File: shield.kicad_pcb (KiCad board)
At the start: 2 copper layers, 56 parts, among them J1 E5V_Conn, J2 V_SERVO_CONN, P1 ROBOT SELECT, P2 CONN_02X10, P3 ENCODER_TRANS, P4 ENCODER_RIGHT, P5 ENCODER_LEFT, P6 5V_CAN_SELECT, P7 GPIO, Q1 Q_PMOS_DGS, U1 ST_Nucleo144_F429ZI_Morpho, U2 SN65HVD256, U3 SN65HVD256, U4 PCA9685

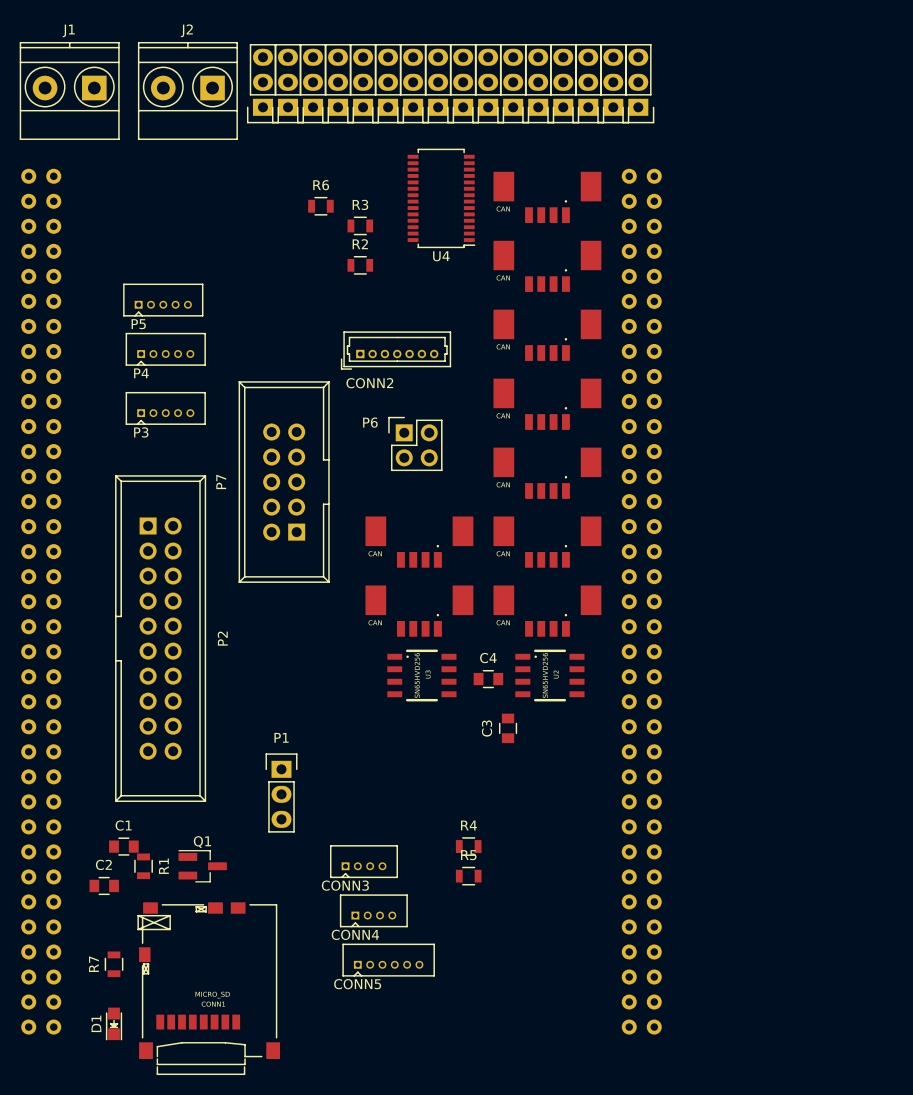
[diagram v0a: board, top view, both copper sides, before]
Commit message: PCB routing
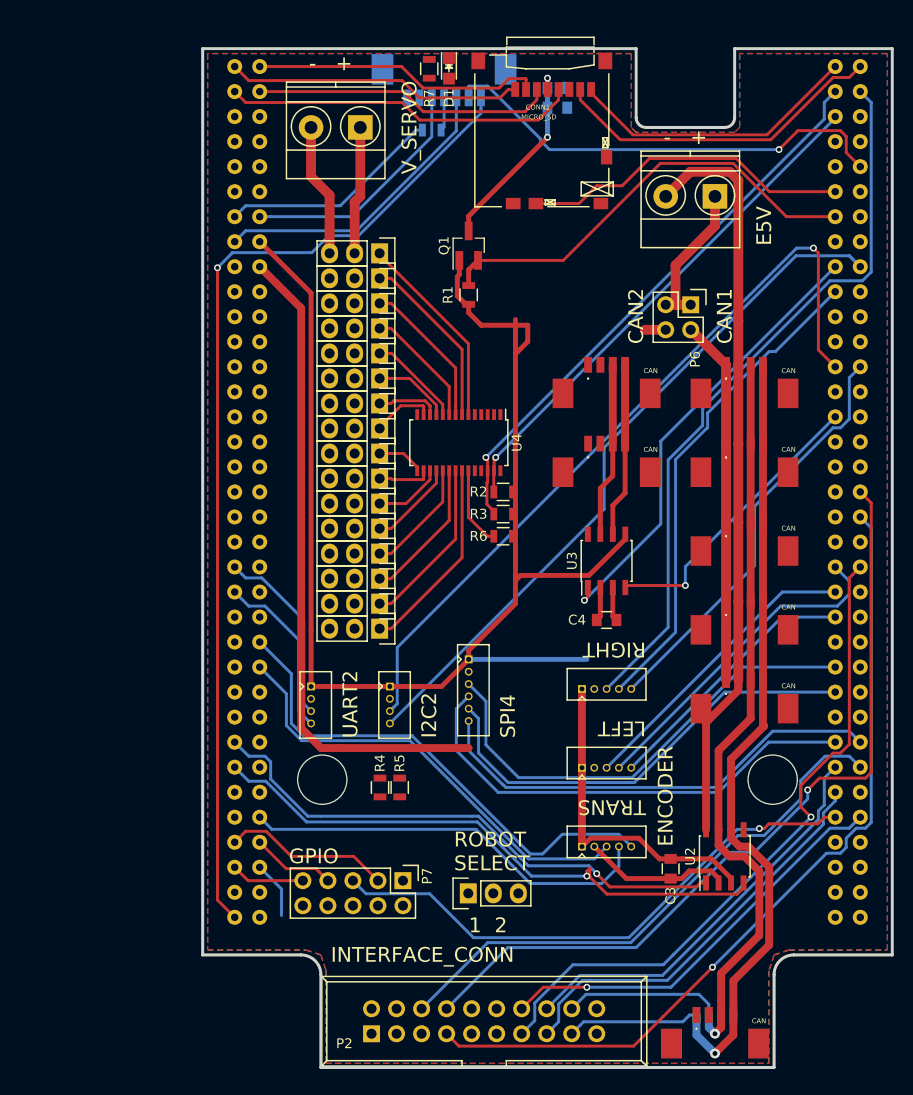
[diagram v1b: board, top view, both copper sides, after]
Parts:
- added R8: 100, Resistors_SMD:R_0805, B.Cu at (88.2, 63.3)
- added _M2: VAL**, _mech:_M2, F.Cu at (122.9, 129.2)
- added _M2: VAL**, _mech:_M2, F.Cu at (77.1, 129.2)
- C1, C2, CONN7: moved to B.Cu
- CONN2: footprint Connectors_Molex:Molex_PicoBlade_53047-0710_07x1.25mm_Straight -> Connectors_Molex:Molex_PicoBlade_53261-0771_07x1.25mm_Angled; moved to B.Cu
- P7: footprint Connect:IDC_Header_Straight_10pins -> Pin_Headers:Pin_Header_Straight_2x05
- U2, U3: footprint _std:_SO-8 -> Housings_SOIC:SOIC-8_3.9x4.9mm_Pitch1.27mm
- moved D1 102.8 mm to (90.0, 57.0), turned to 270 degrees
- moved CONN1 98.8 mm to (96.7, 59.1), turned to 0 degrees
- moved R7 96.4 mm to (88.0, 57.0), turned to 90 degrees
- moved C2 91.4 mm to (101.0, 61.0)
- moved C1 88.7 mm to (101.0, 59.0)
- moved CONN7 81.8 mm to (117.0, 156.0)
- moved CONN8 75.0 mm to (117.0, 156.0), turned to 0 degrees
- moved Q1 68.5 mm to (92.0, 75.0), turned to 90 degrees
- moved R1 66.7 mm to (92.0, 80.0), turned to 90 degrees
- moved P5 65.1 mm to (103.5, 128.0)
- moved J1 64.0 mm to (117.0, 70.0)
- moved P3 62.8 mm to (103.5, 136.0)
- moved P2 56.3 mm to (82.1, 155.0), turned to 0 degrees
- moved P4 56.2 mm to (103.5, 120.0)
- moved CONN30 54.2 mm to (83.0, 113.9), turned to 270 degrees
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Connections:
- CONN2 pad 4: /SWDIO -> Net-(CONN2-Pad4)
- J1 pad 1: GND -> /E5V
- J1 pad 2: /E5V -> GND
- J2 pad 1: GND -> /servo/V_SERVO
- J2 pad 2: /servo/V_SERVO -> GND
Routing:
- net +3.3V: track 0.00 -> 142.3 mm
- net GND: track 0.00 -> 108.1 mm
- net +5V: track 0.00 -> 103.5 mm
- net /DEBUG_UART_RX: track 0.00 -> 101.5 mm, vias 0 -> 1
- net /CAN1L: track 0.00 -> 93.9 mm, vias 0 -> 1
- net /CAN1H: track 0.00 -> 91.9 mm, vias 0 -> 1
- net /EXT_IO_4: track 0.00 -> 85.0 mm, vias 0 -> 1
- net /EXT_IO_5: track 0.00 -> 82.5 mm, vias 0 -> 1
- net /I2C2_SCL: track 0.00 -> 78.8 mm, vias 0 -> 1
- net /ENCODER_RIGHT_CHA: track 0.00 -> 74.2 mm
- net /I2C2_SDA: track 0.00 -> 73.1 mm
- net /EXT_IO_10: track 0.00 -> 68.3 mm, vias 0 -> 1
- net /CAN1_RX: track 0.00 -> 59.2 mm, vias 0 -> 1
- net /I2C1_SCL: track 0.00 -> 58.0 mm, vias 0 -> 1
- net /EXT_IO_3: track 0.00 -> 56.7 mm
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- added copper zone on B.Cu, net GND
- added copper zone on F.Cu, net GND
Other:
- board outline added: 70 x 103.4 mm
- net class Default: trace_width 0.25 -> 0.16; via_dia 0.6 -> 0.7
- rule pad_to_mask_clearance: 0.2 -> 0.15
- rule trace_min: 0.2 -> 0.16
- rule via_min_size: 0.4 -> 0.6
- board text added: "- +"
- board text added: "1 2"
- board text added: "CAN1"
- board text added: "CAN2"
- board text added: "E5V"
- board text added: "ENCODER"
- board text added: "GPIO"
- board text added: "I2C2"
- board text added: "INTERFACE_CONN"
- board text added: "LEFT"
- board text added: "RIGHT"
- board text added: "ROBOT SELECT"
- board text added: "SPI4"
- board text added: "TRANS"
- board text added: "UART2"
- board text added: "V_SERVO"
